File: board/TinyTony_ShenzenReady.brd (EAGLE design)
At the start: 15.5 x 17.4 mm, 12 parts, among them U1 ATTINY85

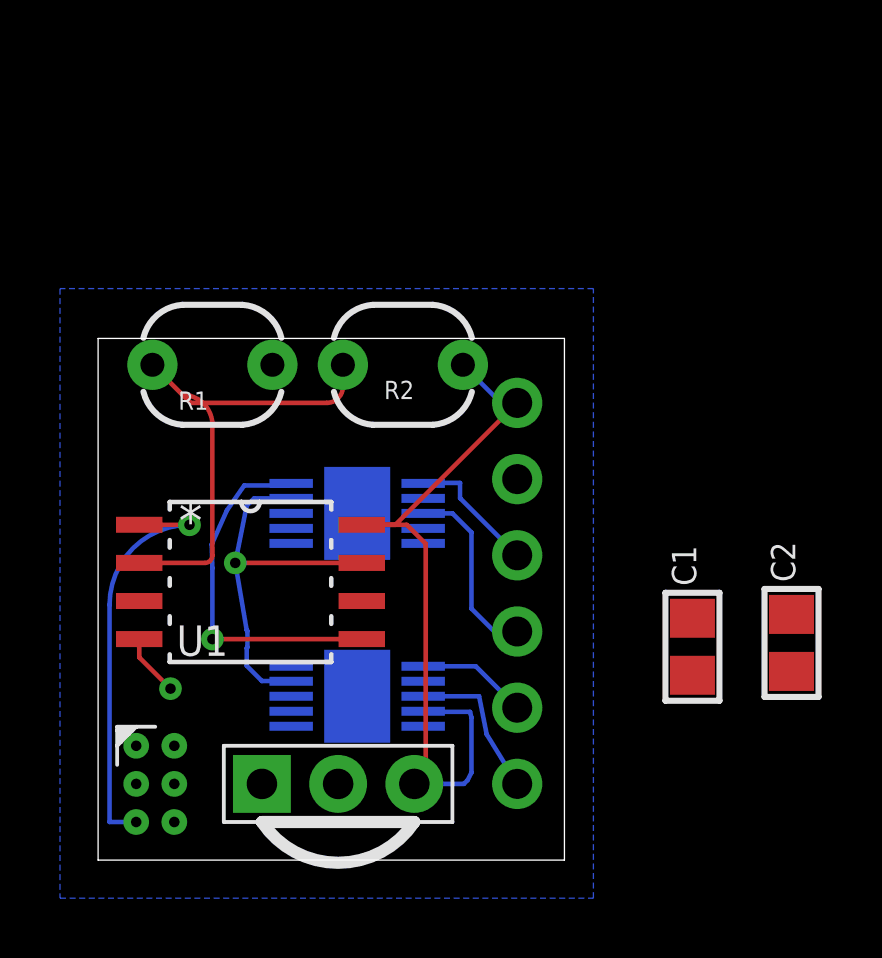
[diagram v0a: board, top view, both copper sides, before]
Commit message: bigger, 1206cp
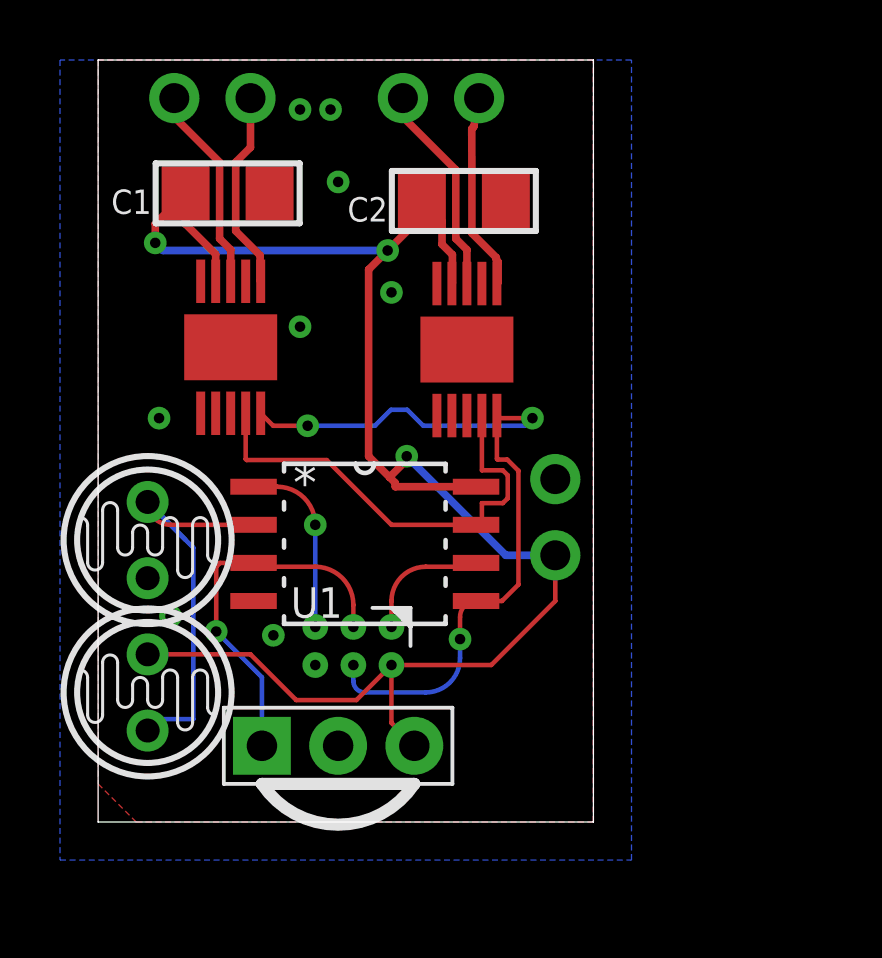
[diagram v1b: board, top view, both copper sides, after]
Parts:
- removed R1, R2: PHOTOCELLPTH, SparkFun-Sensors:PHOTOCELL
- added PHOTOCELL01, PHOTOCELL02: PHOTOCELL0N1, TinyTony_ShenzenReady:TO46-VT200
- C1, C2: device microbuilder:0805_NOTHERMALS -> TinyTony_ShenzenReady:1206
- moved JP2 23.9 mm to (3.81, 24.1), turned to 0 degrees
- moved C1 21.6 mm to (4.32, 21.0), turned to 180 degrees
- moved C2 18.3 mm to (12.2, 20.7), turned to 180 degrees
- moved JP3 16.7 mm to (11.4, 24.1), turned to 0 degrees
- moved U$2 12.4 mm to (4.42, 15.8), flipped to the top, turned to 270 degrees
- moved ISP1 7.03 mm to (7.24, 5.23), turned to 270 degrees
- moved U$3 6.57 mm to (12.3, 15.7), flipped to the top, turned to 270 degrees
- moved U1 4.02 mm to (8.89, 9.27)
- moved JP1 2.84 mm to (15.2, 10.2), turned to 90 degrees
- moved U$1 1.27 mm to (8.00, 2.54)
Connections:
- net 2: now also PHOTOCELL01.1, PHOTOCELL02.2; no longer R1.2, R2.1
- net GND: now also PHOTOCELL01.2; no longer R1.1
- net VCC: now also PHOTOCELL02.1; no longer R2.2
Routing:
- net VCC: track 25.5 -> 57.1 mm, vias 0 -> 3
- net 5: track 12.0 -> 25.6 mm, vias 1 -> 3
- net 3: track 0.00 -> 12.5 mm, vias 0 -> 1
- net 1: track 13.6 -> 5.99 mm
- net 6: track 0.00 -> 4.21 mm
- net N$4: track 3.71 -> 6.66 mm
- net 7: track 12.9 -> 15.4 mm, vias 1 -> 0
- net N$5: track 4.44 -> 6.61 mm
- net GND: track 2.08 -> 0.00 mm, vias 1 -> 8
- net N$3: track 5.10 -> 6.88 mm
- net 2: track 16.1 -> 15.2 mm
- net N$2: track 6.25 -> 7.07 mm
- added copper zone on layer 1, net GND
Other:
- board size 15.5 x 17.4 mm -> 16.5 x 25.4 mm
